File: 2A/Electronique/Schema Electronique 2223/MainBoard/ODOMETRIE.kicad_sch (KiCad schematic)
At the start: 6 parts

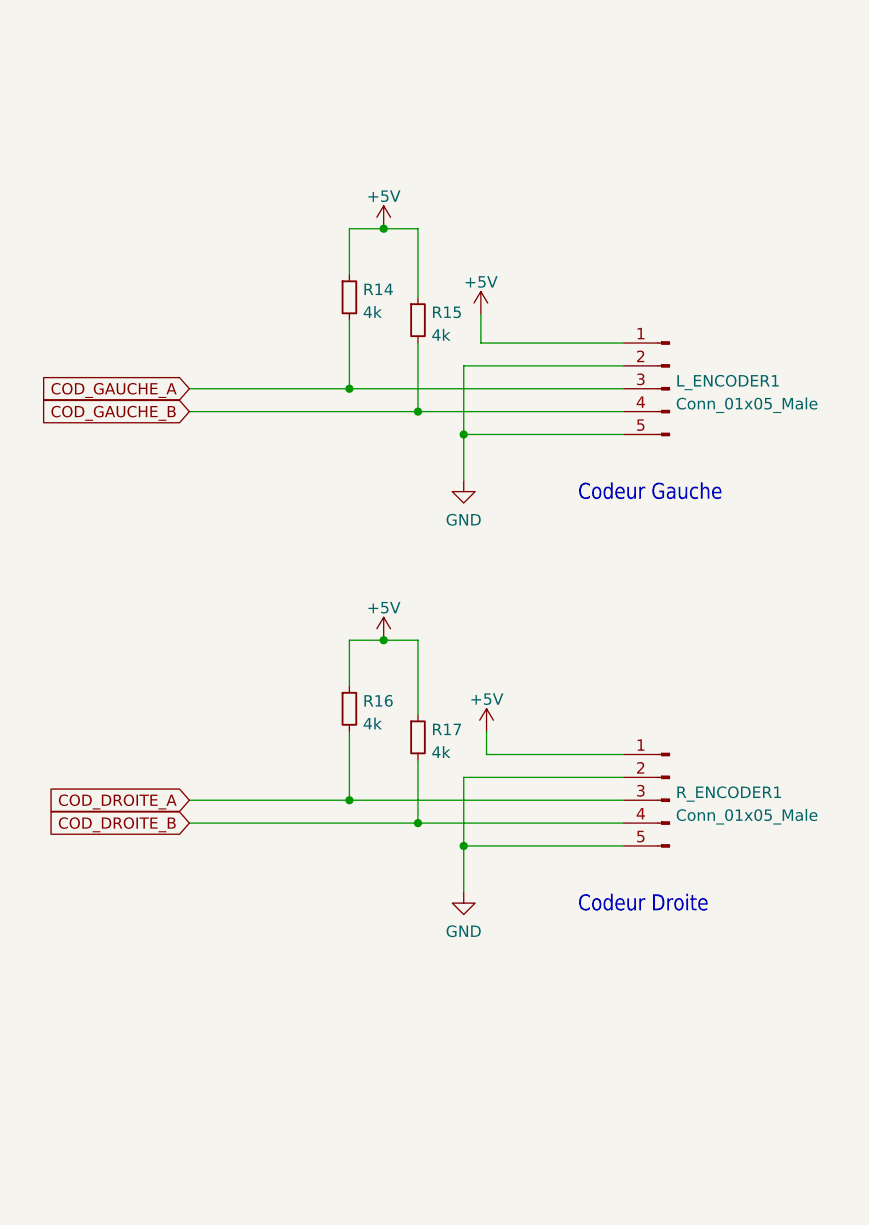
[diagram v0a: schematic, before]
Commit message: schematic and pcb update, added BOM
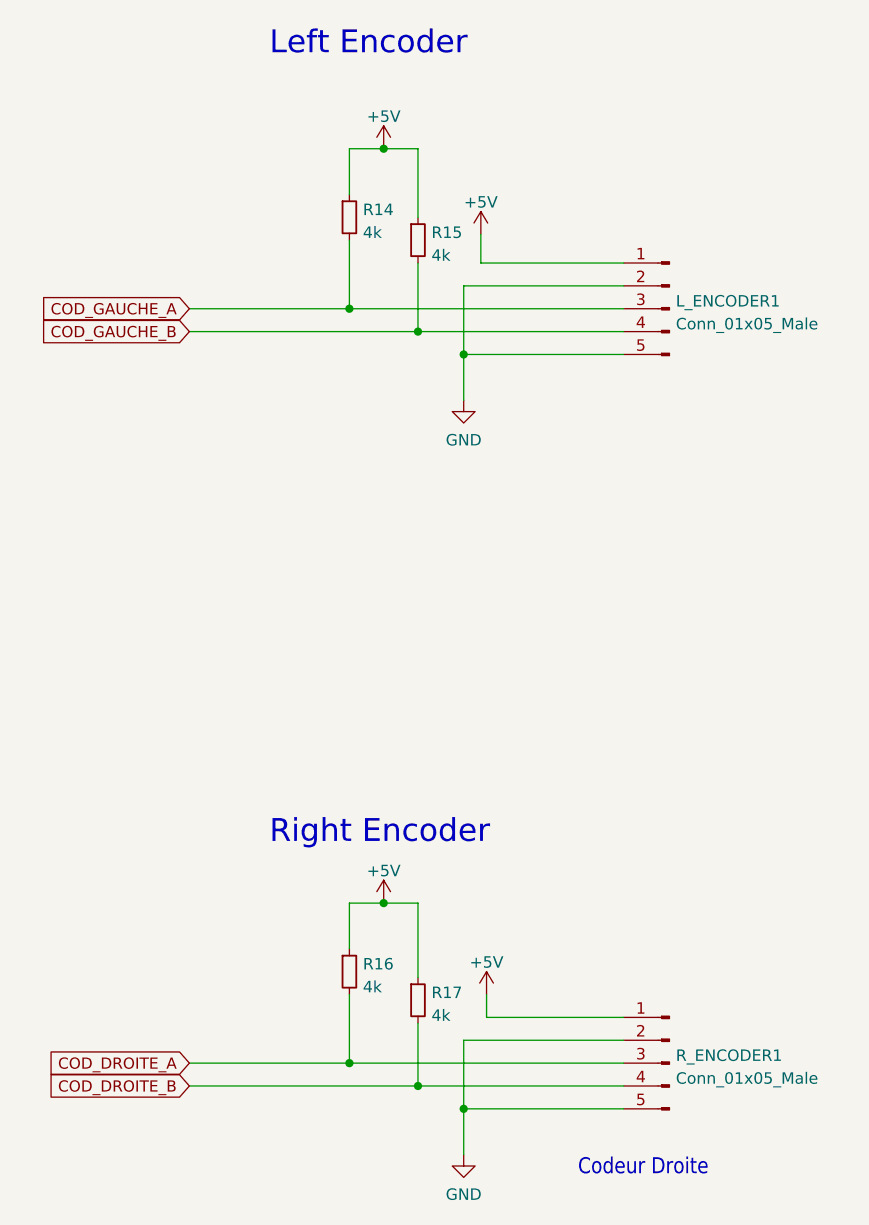
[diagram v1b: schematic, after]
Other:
- note added: "Left Encoder"
- note added: "Right Encoder"
- note removed: "Codeur Gauche"
- moved on the sheet: L_ENCODER1, R14, R15, R16, R17, R_ENCODER1
